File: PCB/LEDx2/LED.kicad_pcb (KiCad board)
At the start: 2 copper layers, 70 x 70 mm, 32 parts, among them J1 Reset, J2 Wago, J3 TC2030-USB-NL-DS, J4 Wago, J5 USB-C-Socket-H, J6 Wago, J7 Wago, T1 T3902_MEMS_Mic, U6 ESP32-S3-MINI-1, U7 MD8942

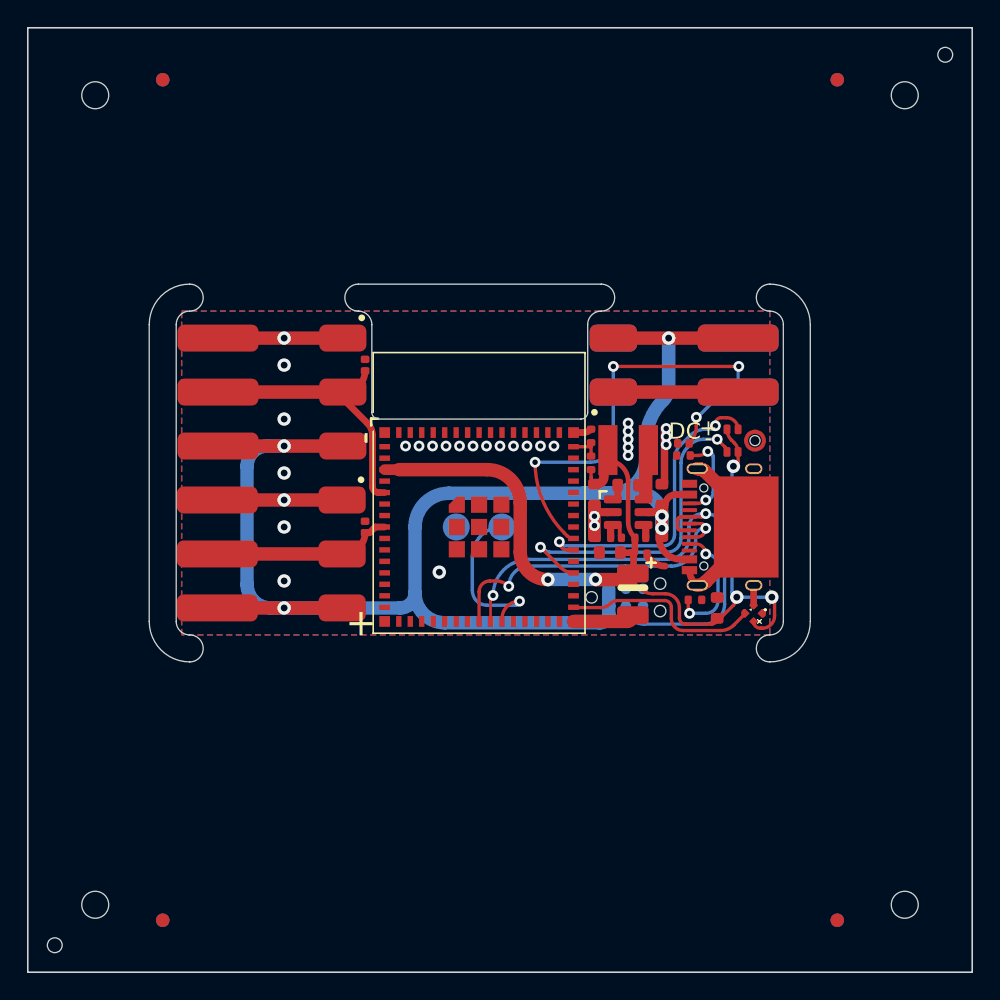
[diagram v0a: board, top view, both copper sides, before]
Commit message: Re-image
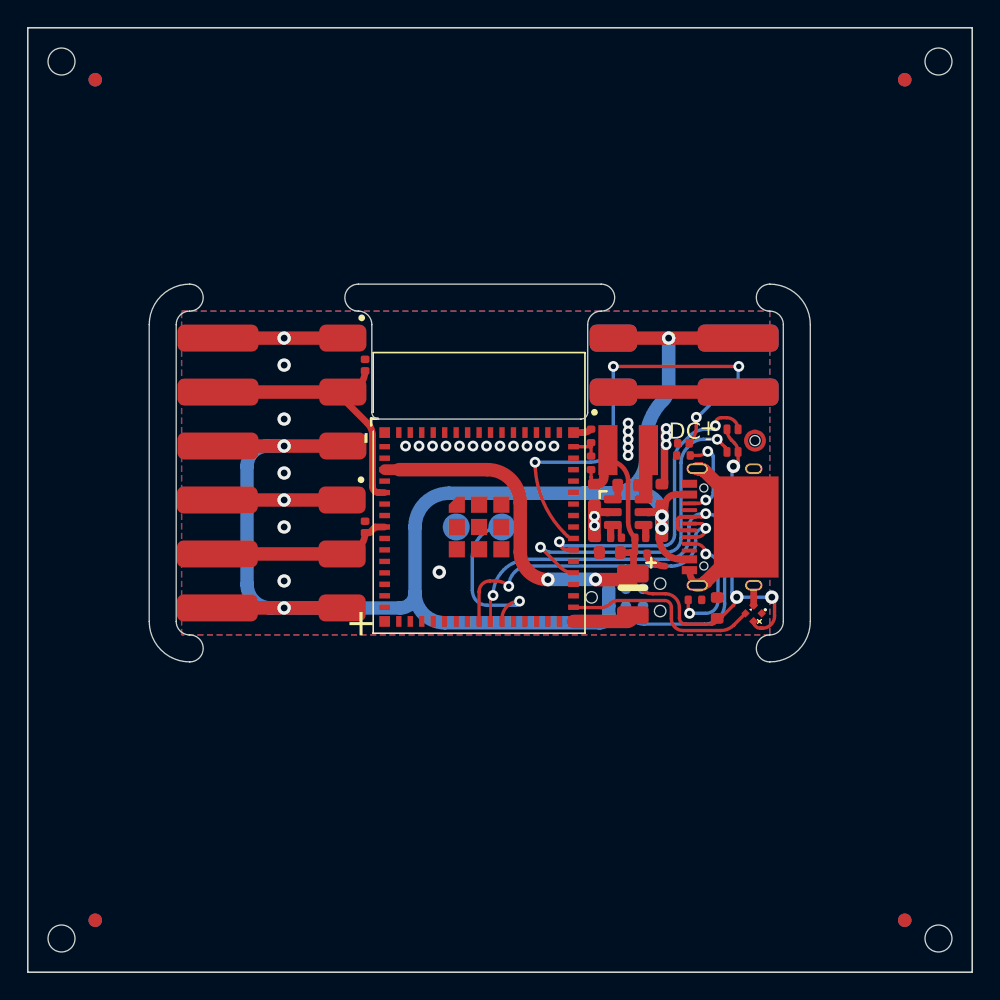
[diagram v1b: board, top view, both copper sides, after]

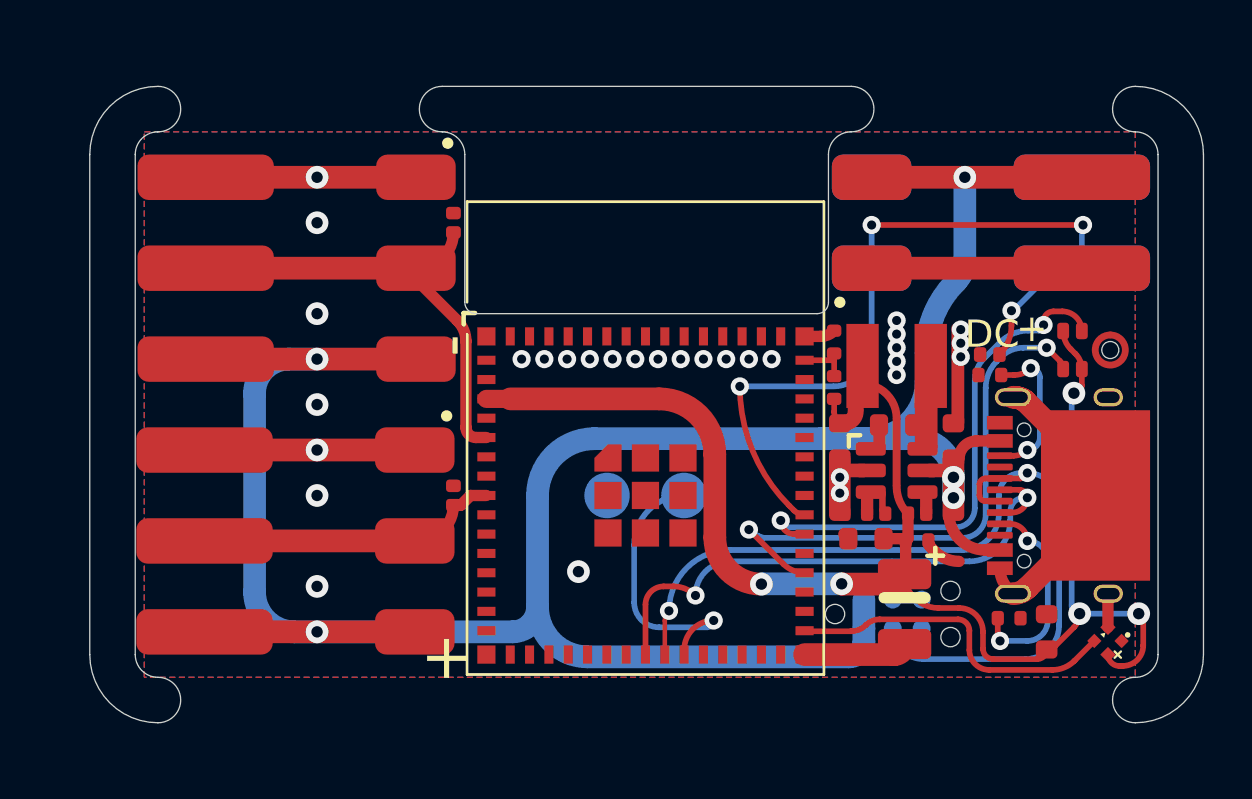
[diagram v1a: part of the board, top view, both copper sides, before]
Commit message: PCB Update
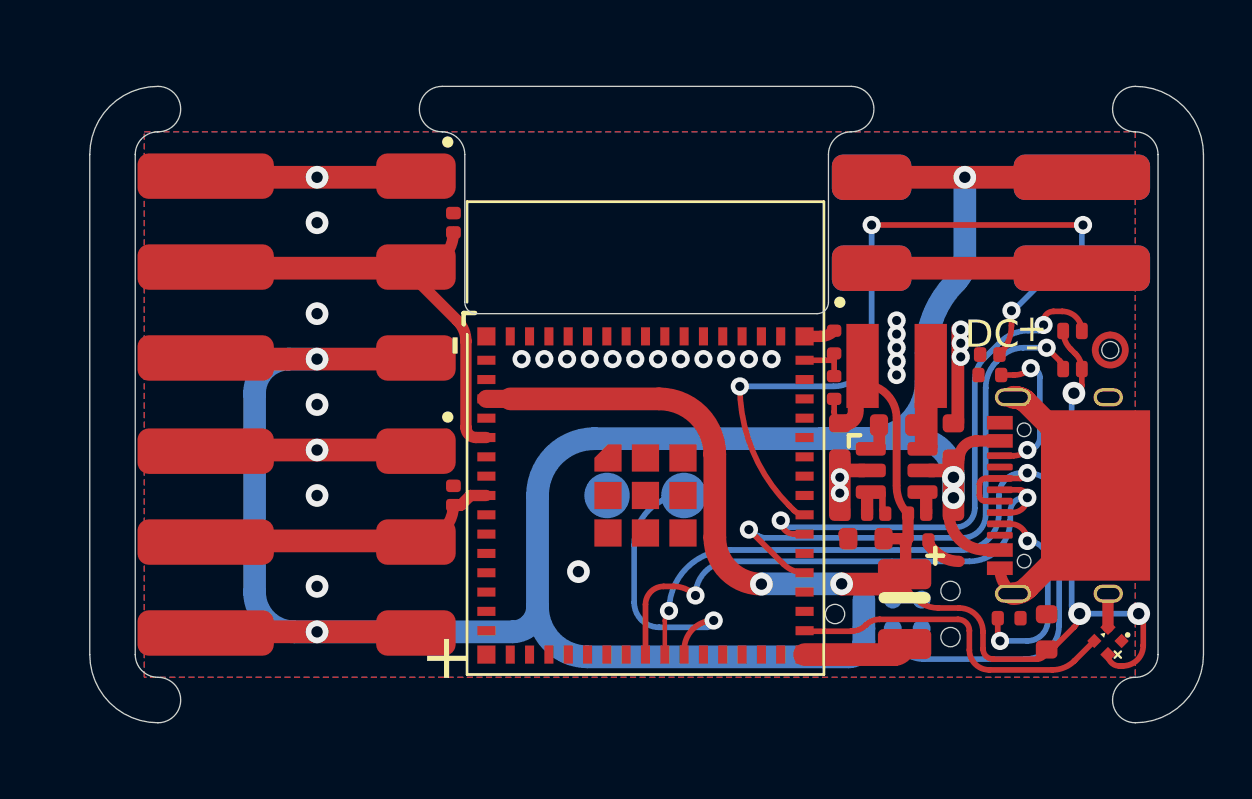
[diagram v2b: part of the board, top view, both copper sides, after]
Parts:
- moved J2 0.07 mm to (83.8, 104.0)
